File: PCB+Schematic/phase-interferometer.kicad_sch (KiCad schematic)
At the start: 63 parts, among them U1 RP2040, U2 ADE-1+, U3 BGA2803, U4 BGA2803, U5 ADE-1+, U6 BGA2803, U7 ADE-1+, U8 W25Q128JVS, Y1 Si5351A-B-GT, Y2 25MHz, Y3 ABM8-272-T3

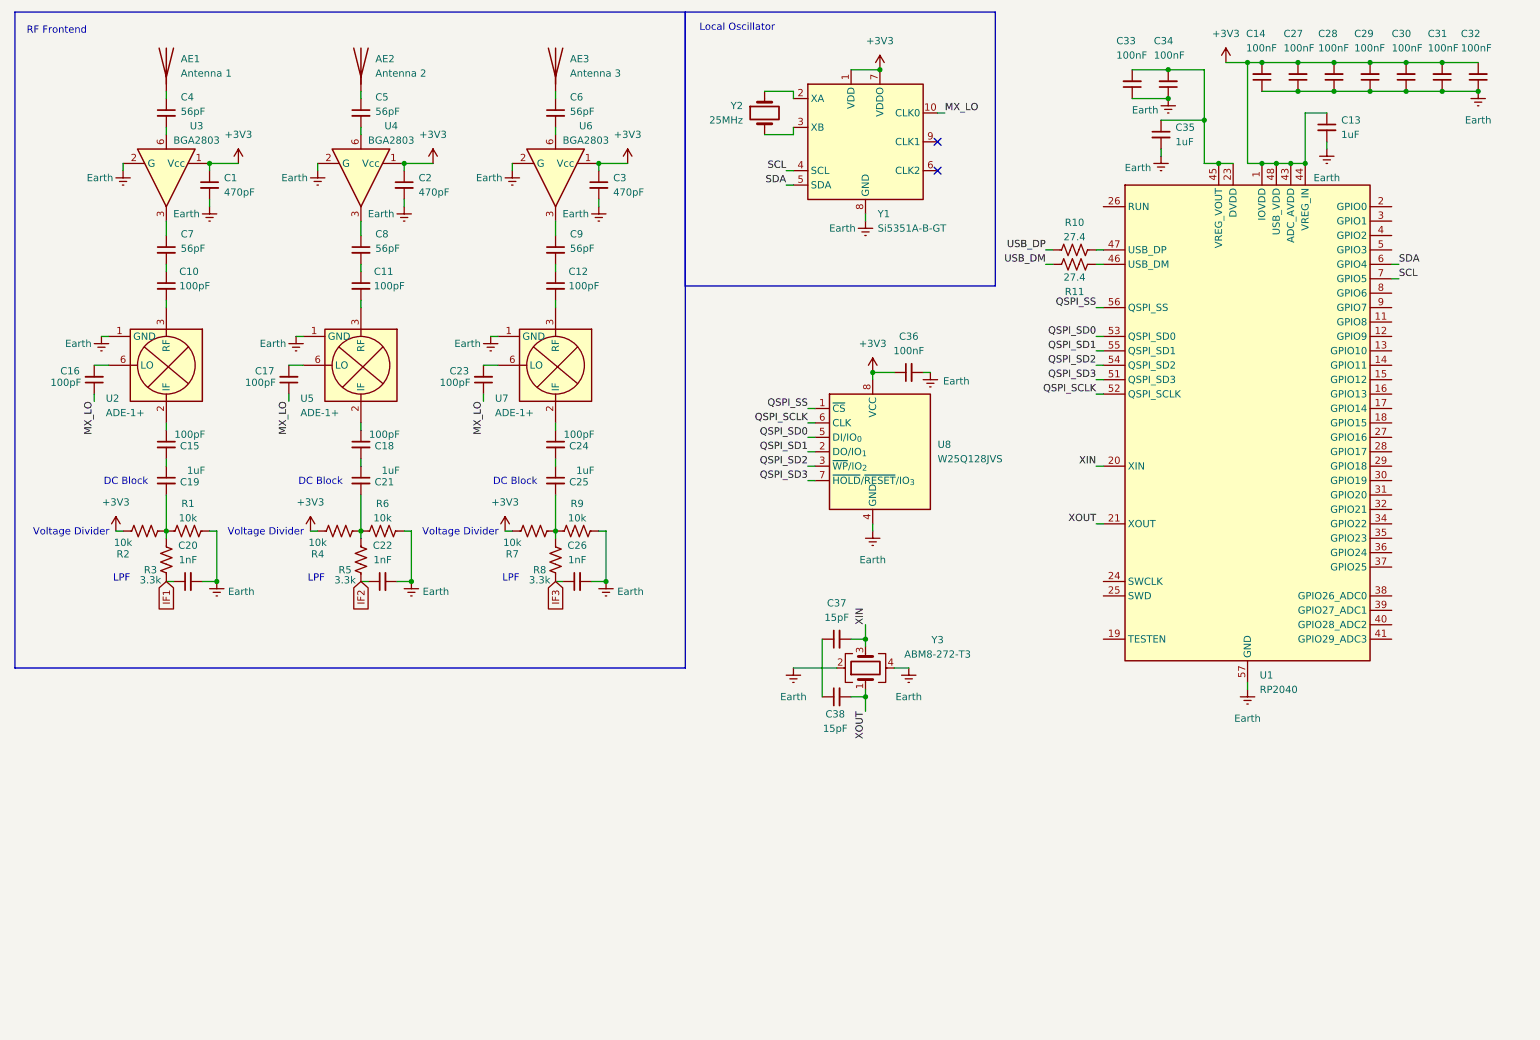
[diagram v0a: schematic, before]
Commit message: finish pcb!
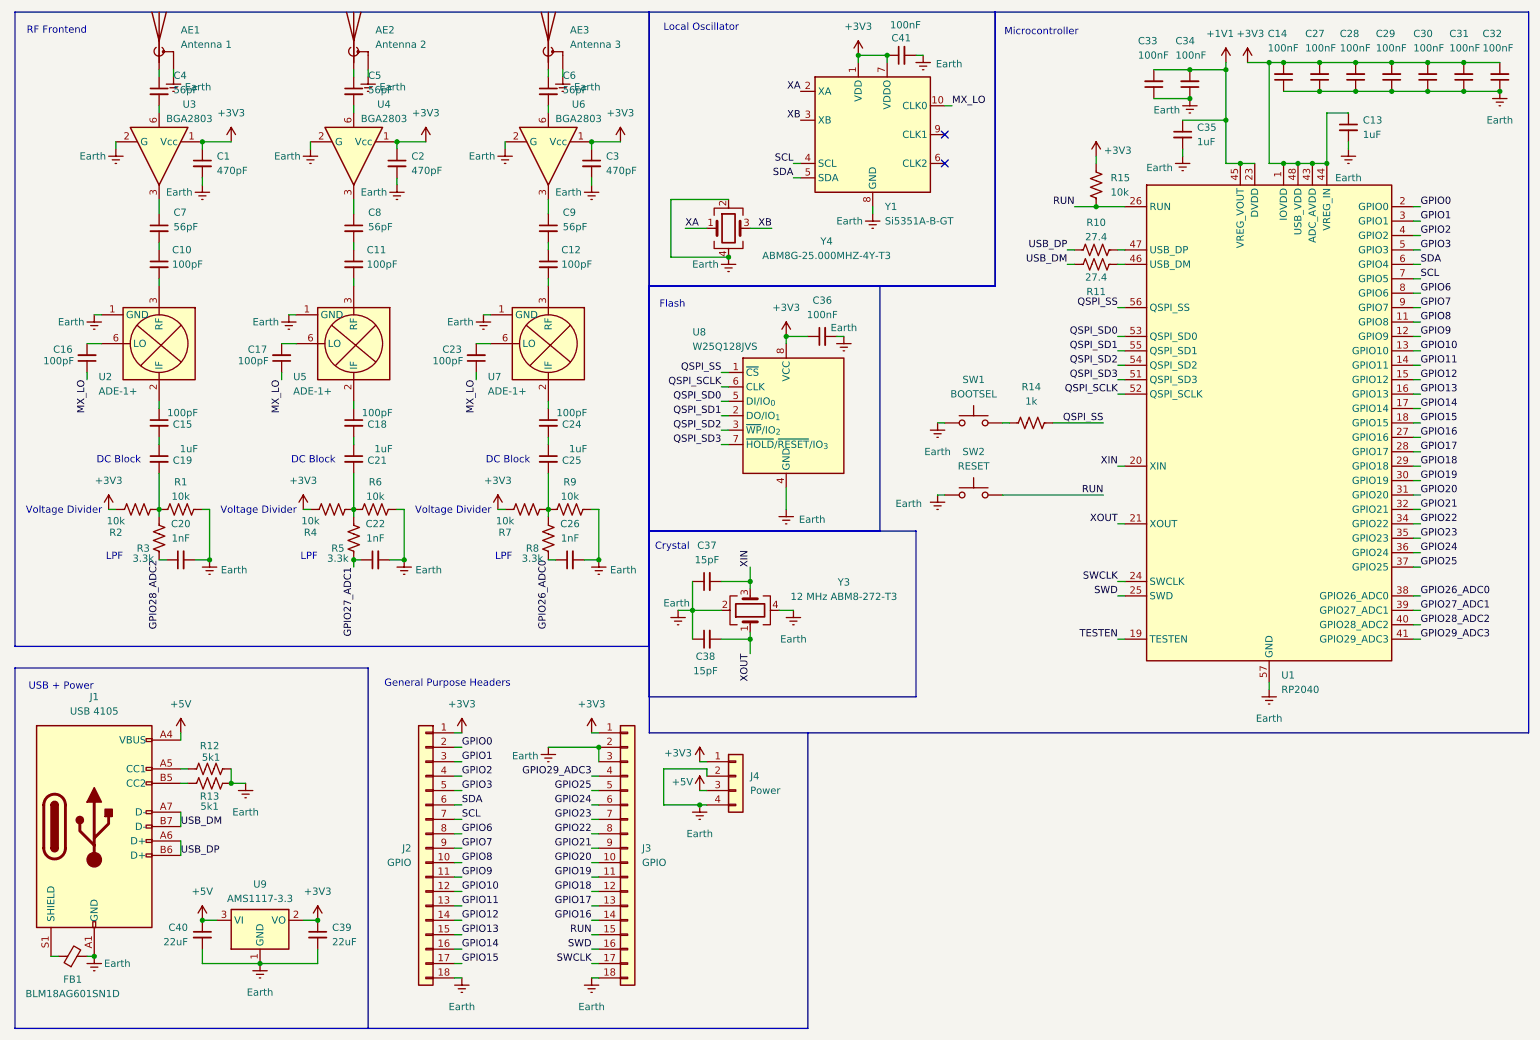
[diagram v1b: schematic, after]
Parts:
- removed Y2: 25MHz, symbol Device:Crystal
- added C39, C40: 22uF, Capacitor_SMD:C_0603_1608Metric, symbol Device:C_Small
- added C41: 100nF, Capacitor_SMD:C_0603_1608Metric, symbol Device:C_Small
- added FB1: BLM18AG601SN1D, Resistor_SMD:R_0201_0603Metric, symbol Device:FerriteBead_Small
- added J1: USB 4105, Connector_USB:USB_C_Receptacle_GCT_USB4105-xx-A_16P_TopMnt_Horizontal, symbol Connector:USB_C_Receptacle_USB2.0_14P
- added J2, J3: GPIO, Connector_PinSocket_2.54mm:PinSocket_1x18_P2.54mm_Vertical, symbol Connector_Generic:Conn_01x18
- added J4: Power, Connector_PinSocket_2.54mm:PinSocket_1x04_P2.54mm_Vertical, symbol Connector_Generic:Conn_01x04
- added R12, R13: 5k1, Resistor_SMD:R_0603_1608Metric, symbol Device:R_US
- added R14: 1k, Resistor_SMD:R_0603_1608Metric, symbol Device:R_US
- added R15: 10k, Resistor_SMD:R_0603_1608Metric, symbol Device:R_US
- added SW1: BOOTSEL, Button_Switch_SMD:SW_Tactile_SPST_NO_Straight_CK_PTS636Sx25SMTRLFS, symbol Switch:SW_Push
- added SW2: RESET, Button_Switch_SMD:SW_Tactile_SPST_NO_Straight_CK_PTS636Sx25SMTRLFS, symbol Switch:SW_Push
- added U9: AMS1117-3.3, Package_TO_SOT_SMD:SOT-223-3_TabPin2, symbol Regulator_Linear:AMS1117-3.3
- added Y4: ABM8G-25.000MHZ-4Y-T3, Crystal:Crystal_SMD_Abracon_ABM8G-4Pin_3.2x2.5mm, symbol Device:Crystal_GND24
- AE1, AE2, AE3: footprint (none) -> Connector_PinSocket_2.54mm:PinSocket_1x02_P2.54mm_Vertical; symbol Device:Antenna -> Device:Antenna_Shield
- C1, C10, C11, C12, C13, C14, C15, C16, C17, C18, C19, C2, C20, C21, C22, C23, C24, C25, C26, C27, C28, C29, C3, C30, C31, C32, C33, C34, C35, C36, C37, C38, C4, C5, C6, C7, C8, C9: footprint (none) -> Capacitor_SMD:C_0603_1608Metric
- R1, R10, R11, R2, R3, R4, R5, R6, R7, R8, R9: footprint (none) -> Resistor_SMD:R_0603_1608Metric
- Y3: value ABM8-272-T3 -> 12 MHz ABM8-272-T3; footprint (none) -> Crystal:Crystal_SMD_Abracon_ABM8G-4Pin_3.2x2.5mm
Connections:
- net IF1 is gone; now on net GPIO28_ADC2: C20.1, R3.1
- net IF2 is gone; now on net GPIO27_ADC1: C22.1, R5.1
- net IF3 is gone; now on net GPIO26_ADC0: C26.1, R8.1
- net +3V3: now also C39.1, C41.1, J2.1 (Pin_1), J3.1 (Pin_1), J4.1 (Pin_1), R15.1, U9.2 (VO)
- net Earth: now also AE1.2 (Shield), AE2.2 (Shield), AE3.2 (Shield), C37.1, C38.1, C39.2, C40.2, C41.2, FB1.2, J1.A1 (GND), J1.A12 (GND), J1.B1 (GND), J1.B12 (GND), J2.18 (Pin_18), J3.18 (Pin_18), J3.2 (Pin_2), J3.3 (Pin_3), J4.2 (Pin_2), J4.4 (Pin_4), R12.2, R13.2, SW1.1, SW2.1, U9.1 (GND), Y4.2, Y4.4
- net QSPI_SS: now also R14.2
- net SCL: now also J2.7 (Pin_7)
- net SDA: now also J2.6 (Pin_6)
- net USB_DM: now also J1.A7 (D-), J1.B7 (D-)
- net USB_DP: now also J1.A6 (D+), J1.B6 (D+)
- net +1V1: now reaches C33.2, C34.2, C35.1, U1.23 (DVDD), U1.45 (VREG_VOUT), U1.50 (DVDD)
- net XA: now reaches Y1.2 (XA)
- net XA: now also Y4.1
- net XB: now reaches Y1.3 (XB)
- net XB: now also Y4.3
- net GPIO8: now reaches U1.11 (GPIO8)
- net GPIO8: now also J2.10 (Pin_10)
- net GPIO9: now reaches U1.12 (GPIO9)
- net GPIO9: now also J2.11 (Pin_11)
- net GPIO10: now reaches U1.13 (GPIO10)
- net GPIO10: now also J2.12 (Pin_12)
- net GPIO11: now reaches U1.14 (GPIO11)
- net GPIO11: now also J2.13 (Pin_13)
- net GPIO12: now reaches U1.15 (GPIO12)
- net GPIO12: now also J2.14 (Pin_14)
- net GPIO13: now reaches U1.16 (GPIO13)
- net GPIO13: now also J2.15 (Pin_15)
- net GPIO14: now reaches U1.17 (GPIO14)
- net GPIO14: now also J2.16 (Pin_16)
- net GPIO15: now reaches U1.18 (GPIO15)
- net GPIO15: now also J2.17 (Pin_17)
- net TESTEN: now reaches U1.19 (TESTEN)
- net GPIO0: now reaches U1.2 (GPIO0)
- net GPIO0: now also J2.2 (Pin_2)
- net SWCLK: now reaches U1.24 (SWCLK)
- net SWCLK: now also J3.17 (Pin_17)
- net SWD: now reaches U1.25 (SWD)
- net SWD: now also J3.16 (Pin_16)
- net RUN: now reaches U1.26 (RUN)
- net RUN: now also J3.15 (Pin_15), R15.2, SW2.2
- net GPIO16: now reaches U1.27 (GPIO16)
- net GPIO16: now also J3.14 (Pin_14)
- net GPIO17: now reaches U1.28 (GPIO17)
- net GPIO17: now also J3.13 (Pin_13)
- net GPIO18: now reaches U1.29 (GPIO18)
- net GPIO18: now also J3.12 (Pin_12)
- net GPIO1: now reaches U1.3 (GPIO1)
- net GPIO1: now also J2.3 (Pin_3)
- net GPIO19: now reaches U1.30 (GPIO19)
- net GPIO19: now also J3.11 (Pin_11)
- net GPIO20: now reaches U1.31 (GPIO20)
- net GPIO20: now also J3.10 (Pin_10)
- net GPIO21: now reaches U1.32 (GPIO21)
- net GPIO21: now also J3.9 (Pin_9)
- net GPIO22: now reaches U1.34 (GPIO22)
- net GPIO22: now also J3.8 (Pin_8)
- net GPIO23: now reaches U1.35 (GPIO23)
- net GPIO23: now also J3.7 (Pin_7)
- net GPIO24: now reaches U1.36 (GPIO24)
- net GPIO24: now also J3.6 (Pin_6)
- net GPIO25: now reaches U1.37 (GPIO25)
- net GPIO25: now also J3.5 (Pin_5)
- net GPIO26_ADC0: now reaches U1.38 (GPIO26_ADC0)
- net GPIO27_ADC1: now reaches U1.39 (GPIO27_ADC1)
- net GPIO2: now reaches U1.4 (GPIO2)
- net GPIO2: now also J2.4 (Pin_4)
- net GPIO28_ADC2: now reaches U1.40 (GPIO28_ADC2)
- net GPIO29_ADC3: now reaches U1.41 (GPIO29_ADC3)
- net GPIO29_ADC3: now also J3.4 (Pin_4)
- net GPIO3: now reaches U1.5 (GPIO3)
- net GPIO3: now also J2.5 (Pin_5)
- net GPIO6: now reaches U1.8 (GPIO6)
- net GPIO6: now also J2.8 (Pin_8)
- net GPIO7: now reaches U1.9 (GPIO7)
- net GPIO7: now also J2.9 (Pin_9)
- new net: J1.A5 (CC1), R12.1
- new net: J1.B5 (CC2), R13.1
- new net: FB1.1, J1.S1 (SHIELD)
- new net: R14.1, SW1.2
- new net +5V: C40.1, J1.A4 (VBUS), J1.A9 (VBUS), J1.B4 (VBUS), J1.B9 (VBUS), J4.3 (Pin_3), U9.3 (VI)
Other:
- note added: "Crystal"
- note added: "Flash"
- note added: "General Purpose Headers"
- note added: "Microcontroller"
- note added: "USB + Power"
- company: (none) -> habtronics
- title: (none) -> Phase Interferometer
- moved on the sheet: C1, C10, C11, C12, C13, C14, C15, C16, C17, C18, C19, C2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
